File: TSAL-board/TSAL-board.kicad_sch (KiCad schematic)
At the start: 74 parts, among them J1 BM02B-PASS-1-TF, J2 19427-0040, J3 BM02B-PASS-1-TF, J4 BM02B-PASS-1-TF, Q1 DMP3098LQ-7, Q2 2N7002K-AU, Q3 2N7002K-AU, Q4 2N7002K-AU, U1 TL431QDBVR, U2 TLP291(GB,SE, U3 TLC555QDRQ1, U4 NCV20071SN2T1G

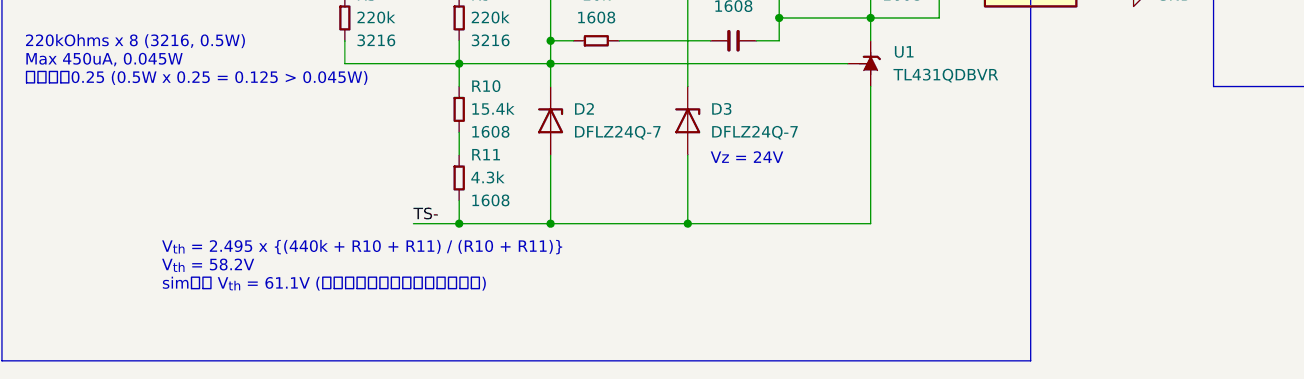
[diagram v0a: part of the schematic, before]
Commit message: sim結果追記
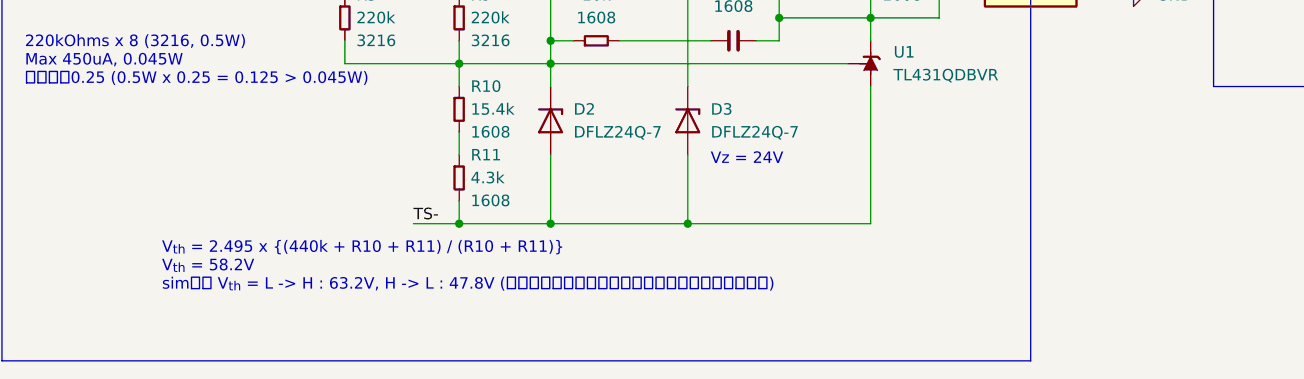
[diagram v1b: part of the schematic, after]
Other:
- note added: "V_{th} = 2.495 x {(440k + R10 + R11) / (R10 + R11)} V_{th} = 58.2V sim結果 V_{th} = L -> H : 63.2V, H -> L : 47.8V (遅れ補償、シュミットトリガ分計算値からズレあり)"
- note removed: "V_{th} = 2.495 x {(440k + R10 + R11) / (R10 + R11)} V_{th} = 58.2V sim結果 V_{th} = 61.1V (遅れ補償分計算値からズレあり)"
